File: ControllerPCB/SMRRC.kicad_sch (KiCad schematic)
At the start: 22 parts, among them J1 Conn_01x08_Socket, J2 Conn_01x05, J3 Conn_01x03, J4 Conn_02x06_Odd_Even, SW1 SW_Push, SW2 SW_Push, U1 THVD1500, U2 PIC16F15345-I/SO, U3 L78L05_SOT89

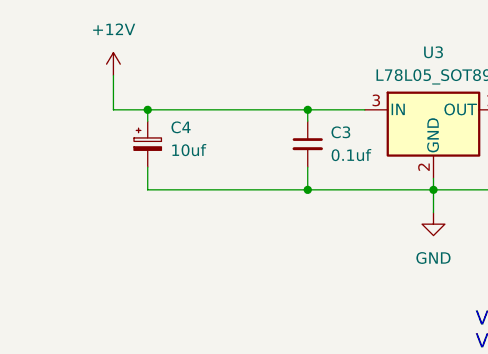
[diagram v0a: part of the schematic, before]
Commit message: USB
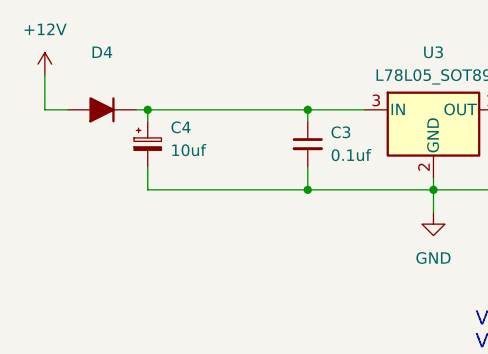
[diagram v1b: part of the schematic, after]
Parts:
- added D4: SMA, Diode_SMD:D_SMA_Handsoldering, symbol Device:D_Filled
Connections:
- net +12V: now also D4.2 (A); no longer C3.1, C4.1, U3.3 (IN)
- new net: C3.1, C4.1, D4.1 (K), U3.3 (IN)
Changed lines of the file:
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@@
 	)
 	(junction
-		(at 48.26 41.91)
+		(at 30.48 33.02)
 		(diameter 0)
 		(color 0 0 0 0)
 	)
 	(junction
-		(at 229.87 33.02)
+		(at 48.26 41.91)
 		(diameter 0)
 		(color 0 0 0 0)
 	)
 	(junction
-		(at 48.26 33.02)
+		(at 229.87 33.02)
 		(diameter 0)
 		(color 0 0 0 0)
 	)
 	(junction
-		(at 222.25 40.64)
+		(at 48.26 33.02)
 		(diameter 0)
 		(color 0 0 0 0)
 	)
 	(junction
-		(at 30.48 33.02)
+		(at 222.25 40.64)
 		(diameter 0)
 		(color 0 0 0 0)
@@
 	(wire
 		(pts
-			(xy 26.67 33.02) (xy 30.48 33.02)
-		)
-		(stroke
-			(width 0)
-			(type default)
-		)
-	)
-	(wire
-		(pts
 			(xy 125.73 38.1) (xy 125.73 49.53)
 		)
@@
 	(wire
 		(pts
-			(xy 26.67 29.21) (xy 26.67 33.02)
+			(xy 29.21 33.02) (xy 30.48 33.02)
 		)
 		(stroke
@@
 	(wire
 		(pts
+			(xy 19.05 33.02) (xy 19.05 29.21)
+		)
+		(stroke
+			(width 0)
+			(type default)
+		)
+	)
+	(wire
+		(pts
 			(xy 170.18 43.18) (xy 170.18 44.45)
 		)
@@
 	(wire
 		(pts
+			(xy 21.59 33.02) (xy 19.05 33.02)
+		)
+		(stroke
+			(width 0)
+			(type default)
+		)
+	)
+	(wire
+		(pts
 			(xy 93.98 97.79) (xy 93.98 92.71)
 		)
@@
 	)
 	(symbol
+		(lib_id "Device:D_Filled")
+		(at 25.4 33.02 180)
+		(unit 1)
+		(exclude_from_sim no)
+		(in_bom yes)
+		(on_board yes)
+		(dnp no)
+		(fields_autoplaced yes)
+		(property "Reference" "D4"
+			(at 25.4 26.67 0)
+			(effects
+				(font
+					(size 1.27 1.27)
+				)
+			)
+		)
+		(property "Value" "SMA"
+			(at 25.4 29.21 0)
+			(effects
+				(font
+					(size 1.27 1.27)
+				)
+				(hide yes)
+			)
+		)
+		(property "Footprint" "Diode_SMD:D_SMA_Handsoldering"
+			(at 25.4 33.02 0)
+			(effects
+				(font
+					(size 1.27 1.27)
+				)
+				(hide yes)
+			)
+		)
+		(property "Datasheet" "~"
+			(at 25.4 33.02 0)
+			(effects
+				(font
+					(size 1.27 1.27)
+				)
+				(hide yes)
+			)
+		)
+		(property "Description" "Diode, filled shape"
+			(at 25.4 33.02 0)
+			(effects
+				(font
+					(size 1.27 1.27)
+				)
+				(hide yes)
+			)
+		)
+		(property "Sim.Device" "D"
+			(at 25.4 33.02 0)
+			(effects
+				(font
+					(size 1.27 1.27)
+				)
+				(hide yes)
+			)
+		)
+		(property "Sim.Pins" "1=K 2=A"
+			(at 25.4 33.02 0)
+			(effects
+				(font
+					(size 1.27 1.27)
+				)
+				(hide yes)
+			)
+		)
+		(pin "1"
+		)
+		(pin "2"
+		)
+		(instances
+			(project ""
+				(path "/256d9eaf-63b3-4e0d-9ae8-9d6979ba55b0"
+					(reference "D4")
+					(unit 1)
+				)
+			)
+		)
+	)
+	(symbol
 		(lib_id "Connector_Generic:Conn_02x06_Odd_Even")
 		(at 161.29 54.61 0)
@@
 	(symbol
 		(lib_id "power:+12V")
-		(at 26.67 29.21 0)
+		(at 19.05 29.21 0)
 		(unit 1)
 		(exclude_from_sim no)
@@
 		(fields_autoplaced yes)
 		(property "Reference" "#PWR06"
-			(at 26.67 33.02 0)
+			(at 19.05 33.02 0)
 			(effects
 				(font
@@
 		)
 		(property "Value" "+12V"
-			(at 26.67 24.13 0)
+			(at 19.05 24.13 0)
 			(effects
 				(font
@@
 		)
 		(property "Footprint" ""
-			(at 26.67 29.21 0)
+			(at 19.05 29.21 0)
 			(effects
 				(font
@@
 		)
 		(property "Datasheet" ""
-			(at 26.67 29.21 0)
+			(at 19.05 29.21 0)
 			(effects
 				(font
@@
 		)
 		(property "Description" "Power symbol creates a global label with name \"+12V\""
-			(at 26.67 29.21 0)
+			(at 19.05 29.21 0)
 			(effects
 				(font
